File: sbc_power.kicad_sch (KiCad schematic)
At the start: 44 parts, among them J10 ATX-24, J14 Conn_01x04, J15 Conn_01x04, J16 Conn_01x04

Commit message: part tweaks, BOM is pretty much finalized, use 0.5W resistors for bleeders
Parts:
- F2, F4, F5: LCSC Part # C92887 -> C3760254; Manufacturer_Name (none) -> Bourns; Manufacturer_Part_Number (none) -> MF-RHT100-0
- F3: LCSC Part # C2687079 -> C3761895; Manufacturer_Name (none) -> Bourns; Manufacturer_Part_Number (none) -> MF-RHT200-0
- J10: LCSC Part # C7541562 -> C587701; Manufacturer_Name (none) -> Molex; Manufacturer_Part_Number (none) -> 44206-0007
- R41, R42, R43, R44: footprint Resistor_SMD:R_0805_2012Metric -> Resistor_SMD:R_1210_3225Metric; LCSC Part # C723424 -> C620660
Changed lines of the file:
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@@
 			)
 		)
-		(property "Description" "LCSC #C92887"
+		(property "Description" "LCSC #C3760254"
 			(at 226.06 25.4 0)
 			(effects
@@
 			)
 		)
-		(property "Manufacturer_Name" ""
+		(property "Manufacturer_Name" "Bourns"
 			(at 226.06 25.4 0)
 			(effects
@@
 			)
 		)
-		(property "Manufacturer_Part_Number" ""
+		(property "Manufacturer_Part_Number" "MF-RHT100-0"
 			(at 226.06 25.4 0)
 			(effects
@@
 			)
 		)
-		(property "LCSC Part #" "C92887"
+		(property "LCSC Part #" "C3760254"
 			(at 226.06 25.4 0)
 			(effects
@@
 			)
 		)
-		(property "Footprint" "Resistor_SMD:R_0805_2012Metric"
+		(property "Footprint" "Resistor_SMD:R_1210_3225Metric"
 			(at 60.706 56.134 90)
 			(effects
@@
 			)
 		)
-		(property "Description" "LCSC #C723424 "
+		(property "Description" "LCSC #C620660"
 			(at 59.69 55.88 0)
 			(effects
@@
 			)
 		)
-		(property "LCSC Part #" "C723424 "
+		(property "LCSC Part #" "C620660"
 			(at 59.69 55.88 0)
 			(effects
@@
 			)
 		)
-		(property "Footprint" "Resistor_SMD:R_0805_2012Metric"
+		(property "Footprint" "Resistor_SMD:R_1210_3225Metric"
 			(at 112.776 165.354 90)
 			(effects
@@
 			)
 		)
-		(property "Description" "LCSC #C723424 "
+		(property "Description" "LCSC #C620660"
 			(at 111.76 165.1 0)
 			(effects
@@
 			)
 		)
-		(property "LCSC Part #" "C723424 "
+		(property "LCSC Part #" "C620660"
 			(at 111.76 165.1 0)
 			(effects
@@
 			)
 		)
-		(property "Footprint" "Resistor_SMD:R_0805_2012Metric"
+		(property "Footprint" "Resistor_SMD:R_1210_3225Metric"
 			(at 125.476 43.434 90)
 			(effects
@@
 			)
 		)
-		(property "Description" "LCSC #C723424 "
+		(property "Description" "LCSC #C620660"
 			(at 124.46 43.18 0)
 			(effects
@@
 			)
 		)
-		(property "LCSC Part #" "C723424 "
+		(property "LCSC Part #" "C620660"
 			(at 124.46 43.18 0)
 			(effects
@@
 			)
 		)
-		(property "Description" "LCSC #C7541562"
+		(property "Description" "LCSC #C587701"
 			(at 146.05 97.79 0)
 			(effects
@@
 			)
 		)
-		(property "Manufacturer_Name" ""
+		(property "Manufacturer_Name" "Molex"
 			(at 146.05 97.79 0)
 			(effects
@@
 			)
 		)
-		(property "Manufacturer_Part_Number" ""
+		(property "Manufacturer_Part_Number" "44206-0007"
 			(at 146.05 97.79 0)
 			(effects
@@
 			)
 		)
-		(property "LCSC Part #" "C7541562"
+		(property "LCSC Part #" "C587701"
 			(at 146.05 97.79 0)
 			(effects
@@
 			)
 		)
-		(property "Footprint" "Resistor_SMD:R_0805_2012Metric"
+		(property "Footprint" "Resistor_SMD:R_1210_3225Metric"
 			(at 98.806 56.134 90)
 			(effects
@@
 			)
 		)
-		(property "Description" "LCSC #C723424 "
+		(property "Description" "LCSC #C620660"
 			(at 97.79 55.88 0)
 			(effects
@@
 			)
 		)
-		(property "LCSC Part #" "C723424 "
+		(property "LCSC Part #" "C620660"
 			(at 97.79 55.88 0)
 			(effects
@@
 			)
 		)
-		(property "Description" "LCSC #C2687079"
+		(property "Description" "LCSC #C3761895"
 			(at 83.82 153.67 0)
 			(effects
@@
 			)
 		)
-		(property "Manufacturer_Name" ""
+		(property "Manufacturer_Name" "Bourns"
 			(at 83.82 153.67 0)
 			(effects
@@
 			)
 		)
-		(property "Manufacturer_Part_Number" ""
+		(property "Manufacturer_Part_Number" "MF-RHT200-0"
 			(at 83.82 153.67 0)
 			(effects
@@
 			)
 		)
-		(property "LCSC Part #" "C2687079"
+		(property "LCSC Part #" "C3761895"
 			(at 83.82 153.67 0)
 			(effects
@@
 			)
 		)
-		(property "Description" "LCSC #C92887"
+		(property "Description" "LCSC #C3760254"
 			(at 77.47 40.64 0)
 			(effects
@@
 			)
 		)
-		(property "Manufacturer_Name" ""
+		(property "Manufacturer_Name" "Bourns"
 			(at 77.47 40.64 0)
 			(effects
@@
 			)
 		)
-		(property "Manufacturer_Part_Number" ""
+		(property "Manufacturer_Part_Number" "MF-RHT100-0"
 			(at 77.47 40.64 0)
 			(effects
@@
 			)
 		)
-		(property "LCSC Part #" "C92887"
+		(property "LCSC Part #" "C3760254"
 			(at 77.47 40.64 0)
 			(effects
@@
 			)
 		)
-		(property "Description" "LCSC #C92887"
+		(property "Description" "LCSC #C3760254"
 			(at 87.63 40.64 0)
 			(effects
@@
 			)
 		)
-		(property "Manufacturer_Name" ""
+		(property "Manufacturer_Name" "Bourns"
 			(at 87.63 40.64 0)
 			(effects
@@
 			)
 		)
-		(property "Manufacturer_Part_Number" ""
+		(property "Manufacturer_Part_Number" "MF-RHT100-0"
 			(at 87.63 40.64 0)
 			(effects
@@
 			)
 		)
-		(property "LCSC Part #" "C92887"
+		(property "LCSC Part #" "C3760254"
 			(at 87.63 40.64 0)
 			(effects

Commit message: minor BOM tweaks due part availability. make some pcb routing a little nicer.
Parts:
- F2, F4, F5: LCSC Part # C3760254 -> C2687078
- F3: LCSC Part # C3761895 -> C2687079
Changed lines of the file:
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@@
 			)
 		)
-		(property "Description" "LCSC #C3760254"
+		(property "Description" "LCSC #C3760254 (Bourns) or LCSC #C2687078"
 			(at 226.06 25.4 0)
 			(effects
@@
 			)
 		)
-		(property "LCSC Part #" "C3760254"
+		(property "LCSC Part #" "C2687078"
 			(at 226.06 25.4 0)
 			(effects
@@
 			)
 		)
-		(property "Description" "LCSC #C3761895"
+		(property "Description" "LCSC #C3761895 (Bourns) or LCSC #C2687079"
 			(at 83.82 153.67 0)
 			(effects
@@
 			)
 		)
-		(property "LCSC Part #" "C3761895"
+		(property "LCSC Part #" "C2687079"
 			(at 83.82 153.67 0)
 			(effects
@@
 			)
 		)
-		(property "Description" "LCSC #C3760254"
+		(property "Description" "LCSC #C3760254 (Bourns) or LCSC #C2687078"
 			(at 77.47 40.64 0)
 			(effects
@@
 			)
 		)
-		(property "LCSC Part #" "C3760254"
+		(property "LCSC Part #" "C2687078"
 			(at 77.47 40.64 0)
 			(effects
@@
 			)
 		)
-		(property "Description" "LCSC #C3760254"
+		(property "Description" "LCSC #C3760254 (Bourns) or LCSC #C2687078"
 			(at 87.63 40.64 0)
 			(effects
@@
 			)
 		)
-		(property "LCSC Part #" "C3760254"
+		(property "LCSC Part #" "C2687078"
 			(at 87.63 40.64 0)
 			(effects

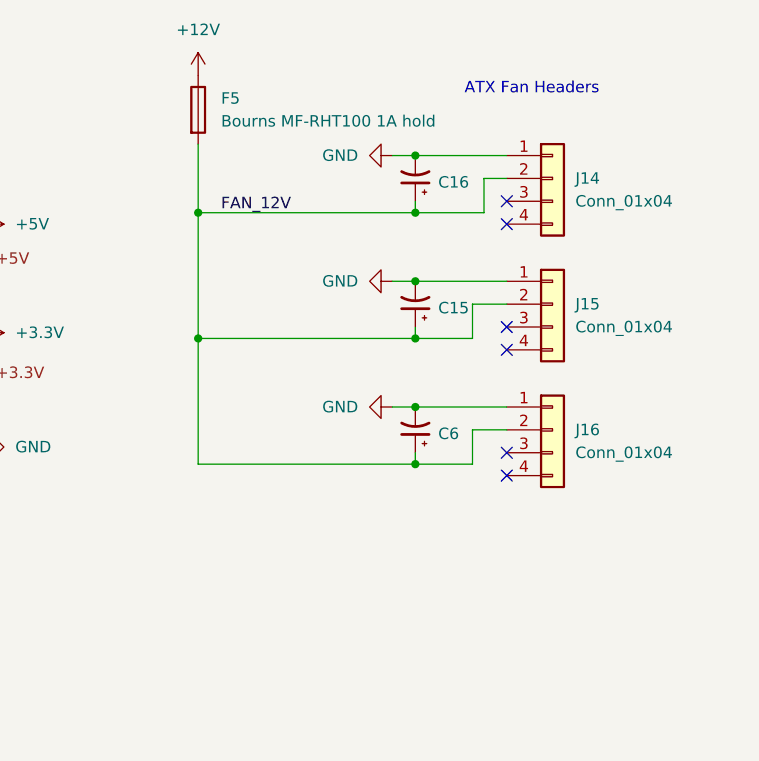
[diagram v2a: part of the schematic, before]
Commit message: routing tweaks, use identity comparator instead of OR gates for IO decode
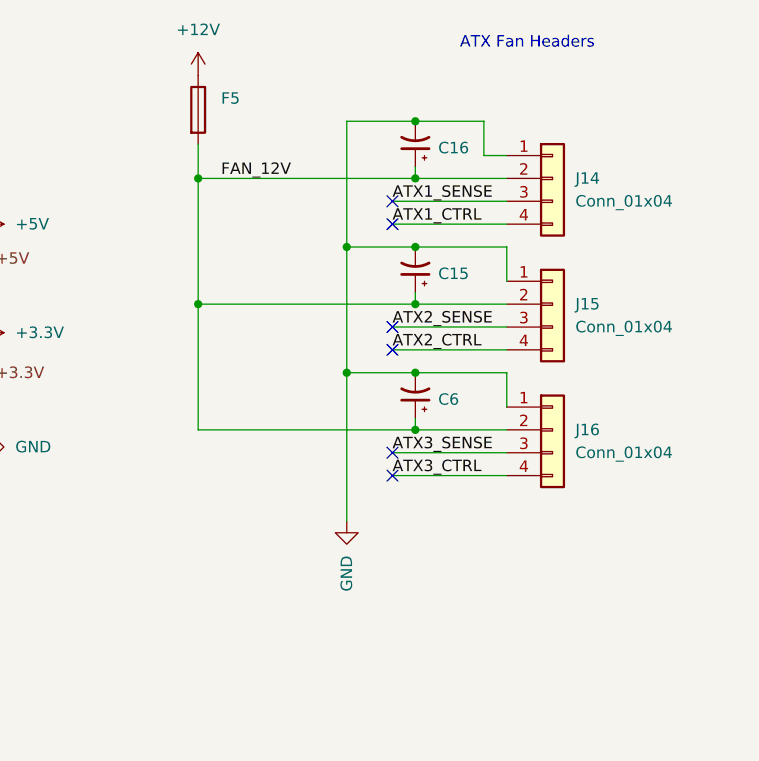
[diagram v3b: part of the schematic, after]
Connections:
- net ATX3_SENSE: now reaches J16.3 (Pin_3)
- net ATX3_CTRL: now reaches J16.4 (Pin_4)
- net ATX2_SENSE: now reaches J15.3 (Pin_3)
- net ATX2_CTRL: now reaches J15.4 (Pin_4)
- net ATX1_SENSE: now reaches J14.3 (Pin_3)
- net ATX1_CTRL: now reaches J14.4 (Pin_4)
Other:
- moved on the sheet: C15, C16, C6
